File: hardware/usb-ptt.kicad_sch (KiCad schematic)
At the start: 0 parts

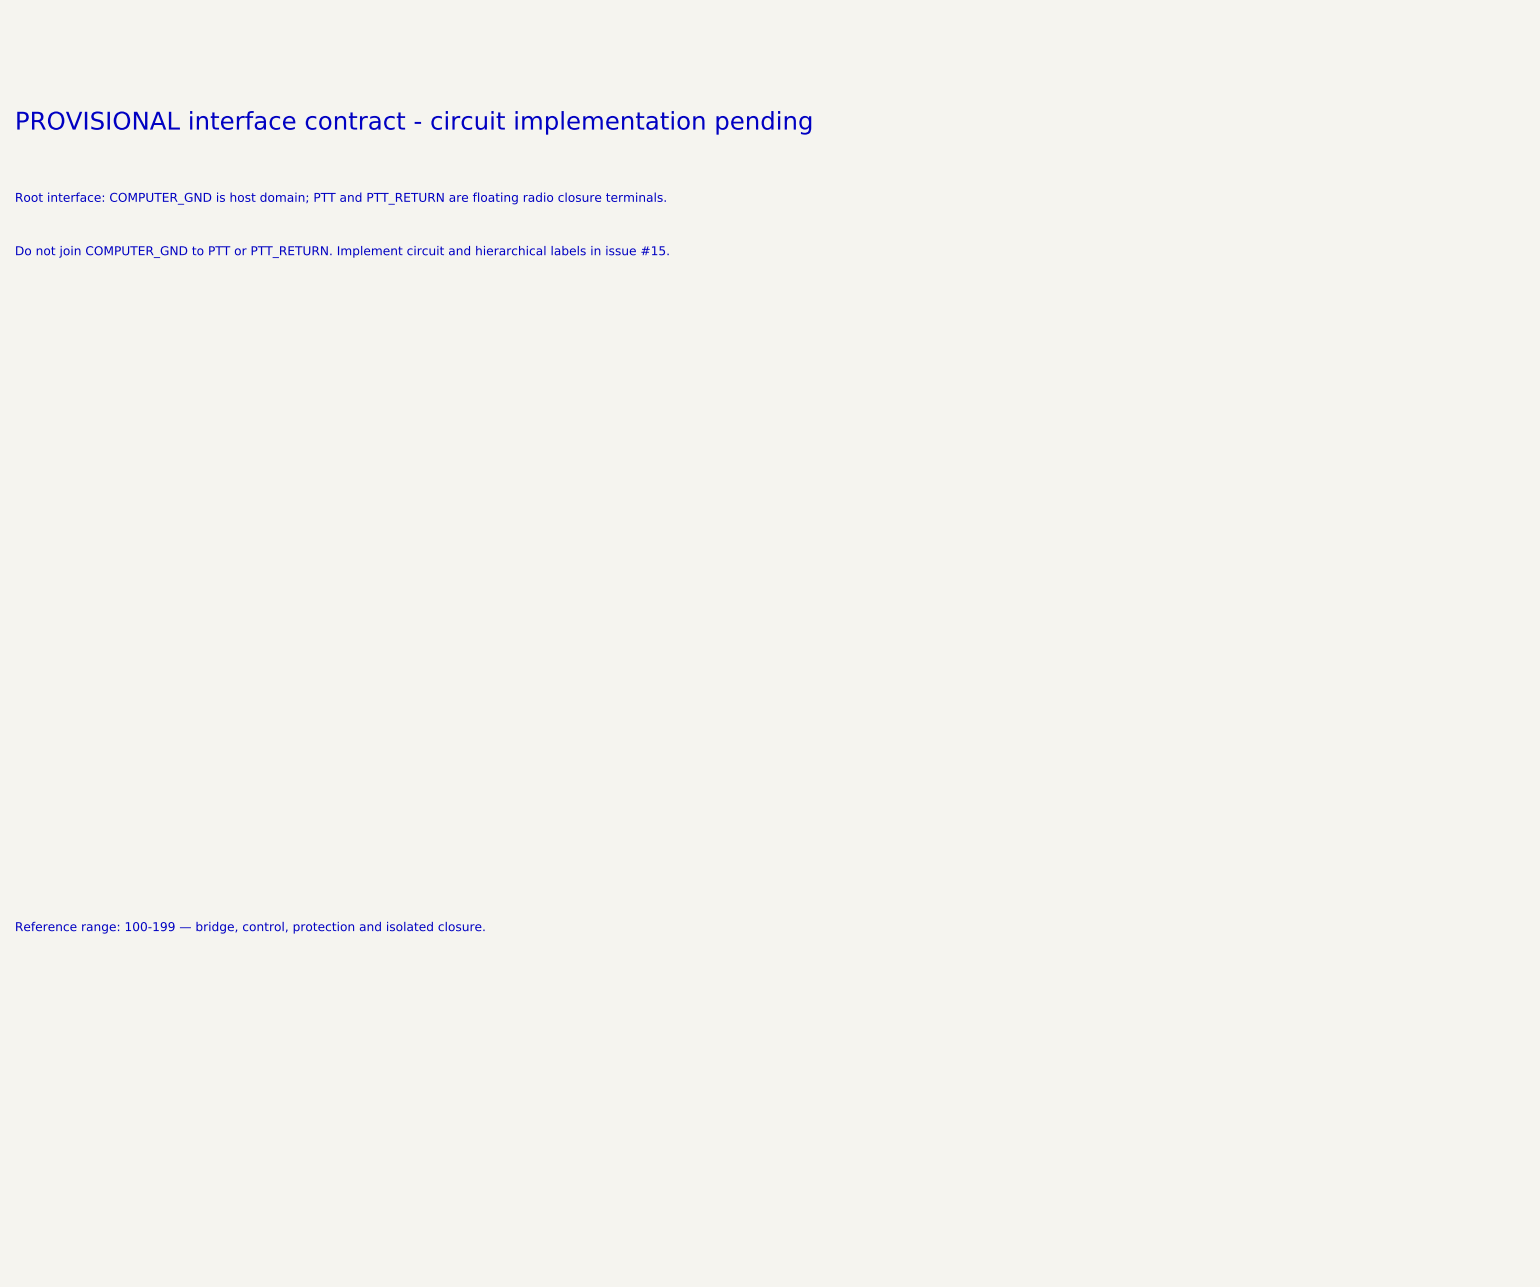
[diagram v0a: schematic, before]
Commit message: Add provisional USB and isolated PTT circuit contract
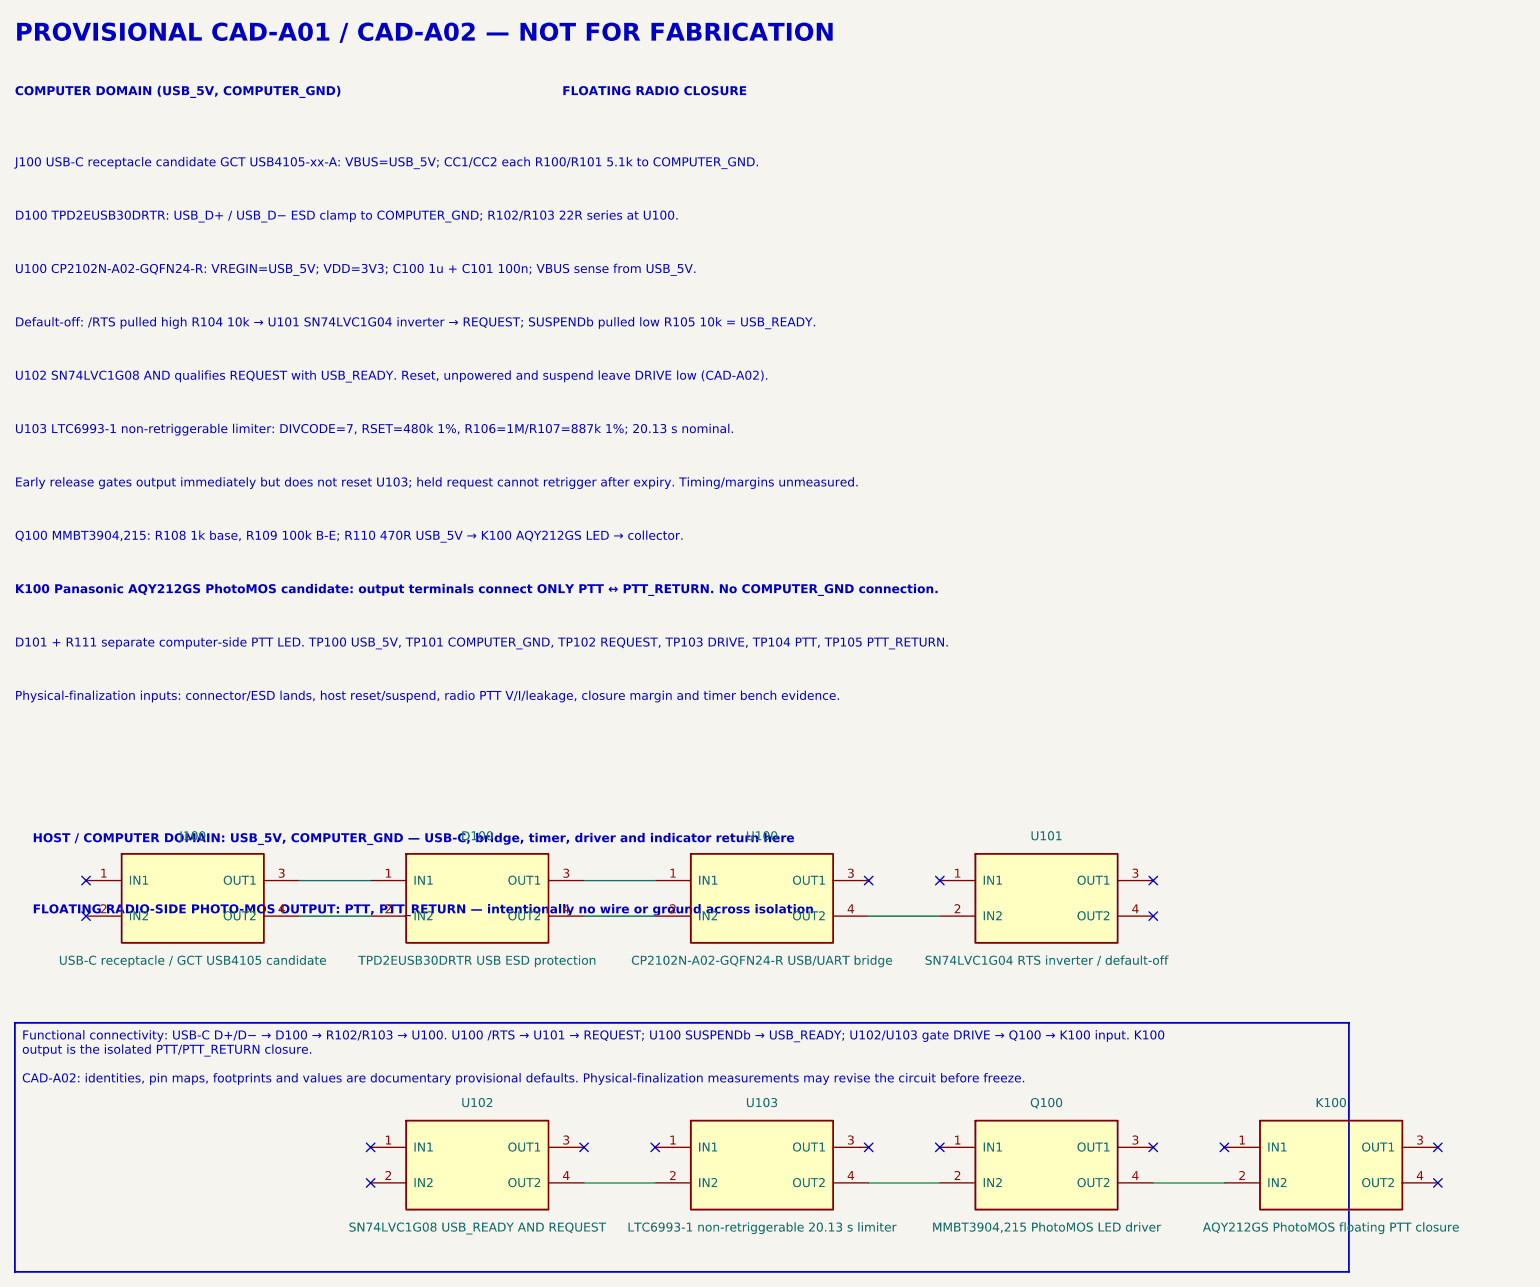
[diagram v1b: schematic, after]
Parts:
- added D100: TPD2EUSB30DRTR USB ESD protection, symbol TS700:PTT_Block
- added J100: USB-C receptacle / GCT USB4105 candidate, symbol TS700:PTT_Block
- added K100: AQY212GS PhotoMOS floating PTT closure, symbol TS700:PTT_Block
- added Q100: MMBT3904,215 PhotoMOS LED driver, symbol TS700:PTT_Block
- added U100: CP2102N-A02-GQFN24-R USB/UART bridge, symbol TS700:PTT_Block
- added U101: SN74LVC1G04 RTS inverter / default-off, symbol TS700:PTT_Block
- added U102: SN74LVC1G08 USB_READY AND REQUEST, symbol TS700:PTT_Block
- added U103: LTC6993-1 non-retriggerable 20.13 s limiter, symbol TS700:PTT_Block
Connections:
- new net: D100.1 (IN1), J100.3 (OUT1)
- new net: D100.2 (IN2), J100.4 (OUT2)
- new net: D100.3 (OUT1), U100.1 (IN1)
- new net: D100.4 (OUT2), U100.2 (IN2)
- new net: U100.4 (OUT2), U101.2 (IN2)
- new net: U102.4 (OUT2), U103.2 (IN2)
- new net: Q100.2 (IN2), U103.4 (OUT2)
- new net: K100.2 (IN2), Q100.4 (OUT2)
- no-connect marks 0 -> 16
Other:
- note added: "COMPUTER DOMAIN (USB_5V, COMPUTER_GND) FLOATING RADIO CLOSURE"
- note added: "D100 TPD2EUSB30DRTR: USB_D+ / USB_D− ESD clamp to COMPUTER_GND; R102/R103 22R series at U100."
- note added: "D101 + R111 separate computer-side PTT LED. TP100 USB_5V, TP101 COMPUTER_GND, TP102 REQUEST, TP103 DRIVE, TP104 PTT, TP105 PTT_RETURN."
- note added: "Default-off: /RTS pulled high R104 10k → U101 SN74LVC1G04 inverter → REQUEST; SUSPENDb pulled low R105 10k = USB_READY."
- note added: "Early release gates output immediately but does not reset U103; held request cannot retrigger after expiry. Timing/margins unmeasured."
- note added: "FLOATING RADIO-SIDE PHOTO-MOS OUTPUT: PTT, PTT_RETURN — intentionally no wire or ground across isolation"
- note added: "HOST / COMPUTER DOMAIN: USB_5V, COMPUTER_GND — USB-C, bridge, timer, driver and indicator return here"
- note added: "J100 USB-C receptacle candidate GCT USB4105-xx-A: VBUS=USB_5V; CC1/CC2 each R100/R101 5.1k to COMPUTER_GND."
- note added: "K100 Panasonic AQY212GS PhotoMOS candidate: output terminals connect ONLY PTT ↔ PTT_RETURN. No COMPUTER_GND connection."
- note added: "PROVISIONAL CAD-A01 / CAD-A02 — NOT FOR FABRICATION"
- note added: "Physical-finalization inputs: connector/ESD lands, host reset/suspend, radio PTT V/I/leakage, closure margin and timer bench evidence."
- note added: "Q100 MMBT3904,215: R108 1k base, R109 100k B-E; R110 470R USB_5V → K100 AQY212GS LED → collector."
- note added: "U100 CP2102N-A02-GQFN24-R: VREGIN=USB_5V; VDD=3V3; C100 1u + C101 100n; VBUS sense from USB_5V."
- note added: "U102 SN74LVC1G08 AND qualifies REQUEST with USB_READY. Reset, unpowered and suspend leave DRIVE low (CAD-A02)."
- note added: "U103 LTC6993-1 non-retriggerable limiter: DIVCODE=7, RSET=480k 1%, R106=1M/R107=887k 1%; 20.13 s nominal."
- note removed: "Do not join COMPUTER_GND to PTT or PTT_RETURN. Implement circuit and hierarchical labels in issue #15."
- note removed: "PROVISIONAL interface contract - circuit implementation pending"
- note removed: "Reference range: 100-199 — bridge, control, protection and isolated closure."
- note removed: "Root interface: COMPUTER_GND is host domain; PTT and PTT_RETURN are floating radio closure terminals."
- title: USB-C and isolated PTT -> USB-C serial and isolated PTT — PROVISIONAL
